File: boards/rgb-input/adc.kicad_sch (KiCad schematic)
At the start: 6 parts, among them U13 MCP1502, U2 MCP3208

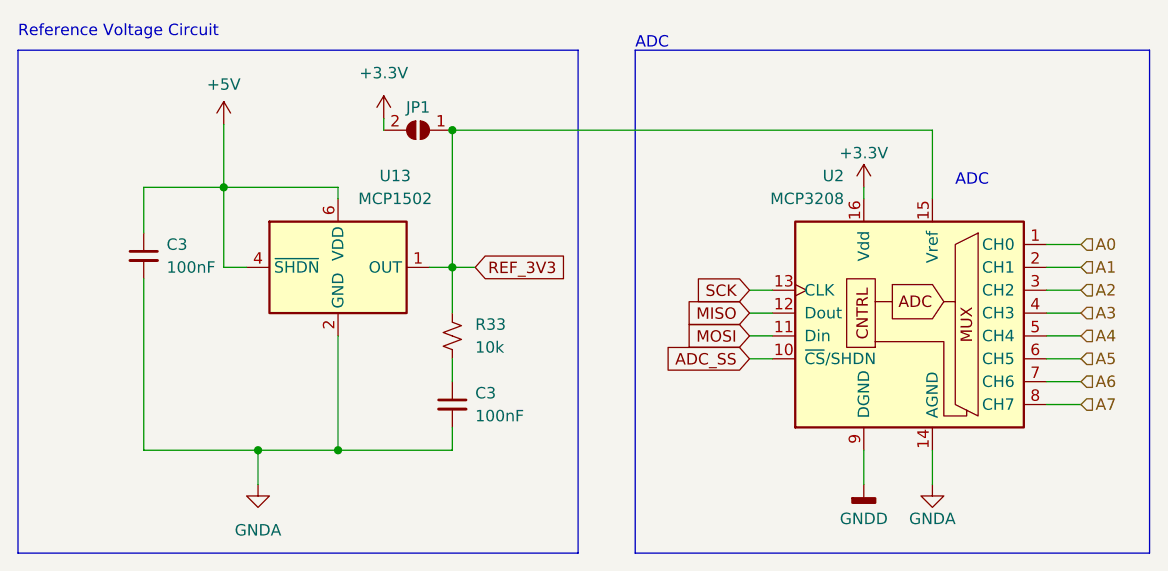
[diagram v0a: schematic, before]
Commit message: more BOM updates.
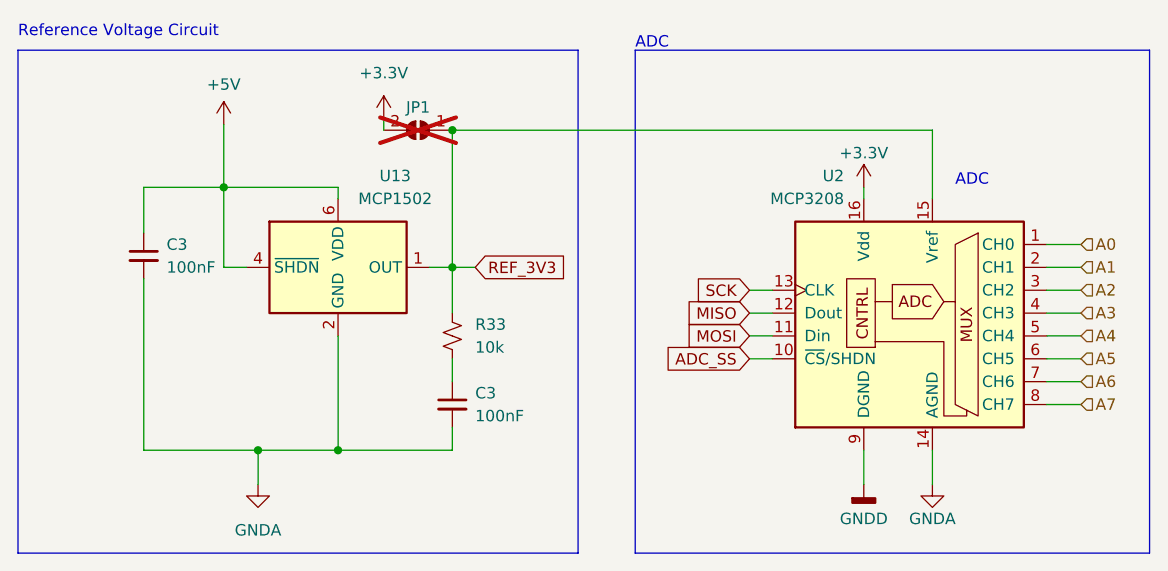
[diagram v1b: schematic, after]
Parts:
- C3: Vendor C0805C102J1HACTU -> (none)
- JP1: now not fitted; now left out of the parts list
- R33: Vendor 652-CR0805JW-104ELF -> (none)
- U13: Mouser (none) -> 579-MCP1502T-33E/CHY
- U2: Mouser (none) -> 579-MCP3208T-BI/SL; Vendor MCP3208T-BI/SL -> (none)
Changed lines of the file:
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@@
       (effects (font (size 1.27 1.27)) hide)
     )
-    (property "Vendor" "MCP3208T-BI/SL" (at 134.62 87.63 0)
+    (property "Mouser" "579-MCP3208T-BI/SL" (at 134.62 87.63 0)
       (effects (font (size 1.27 1.27)) hide)
     )
@@
       (effects (font (size 1.27 1.27)) hide)
     )
-    (property "Vendor" "652-CR0805JW-104ELF" (at 83.82 90.17 0)
-      (effects (font (size 1.27 1.27)) hide)
-    )
     (pin "1")
     (pin "2")
@@
     )
     (property "Datasheet" "http://ww1.microchip.com/downloads/en/DeviceDoc/20005474E.pdf" (at 71.12 82.55 0)
+      (effects (font (size 1.27 1.27)) hide)
+    )
+    (property "Mouser" "579-MCP1502T-33E/CHY" (at 71.12 82.55 0)
       (effects (font (size 1.27 1.27)) hide)
     )
@@
       (effects (font (size 1.27 1.27)) hide)
     )
-    (property "Vendor" "C0805C102J1HACTU" (at 83.82 97.79 0)
-      (effects (font (size 1.27 1.27)) hide)
-    )
     (pin "1")
     (pin "2")
@@
   )
   (symbol (lib_id "Jumper:SolderJumper_2_Open") (at 80.01 67.31 180) (unit 1)
-    (in_bom yes) (on_board yes) (dnp no)
+    (in_bom no) (on_board yes) (dnp yes)
     (property "Reference" "JP1" (at 80.01 64.77 0)
       (effects (font (size 1.27 1.27)))
@@
       (effects (font (size 1.27 1.27)) hide)
     )
-    (property "Vendor" "C0805C102J1HACTU" (at 49.53 81.28 0)
-      (effects (font (size 1.27 1.27)) hide)
-    )
